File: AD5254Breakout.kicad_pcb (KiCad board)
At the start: 2 copper layers, 20.6 x 18 mm, 13 parts, among them J1 Conn_01x08, J2 Conn_01x08, U1 AD5254

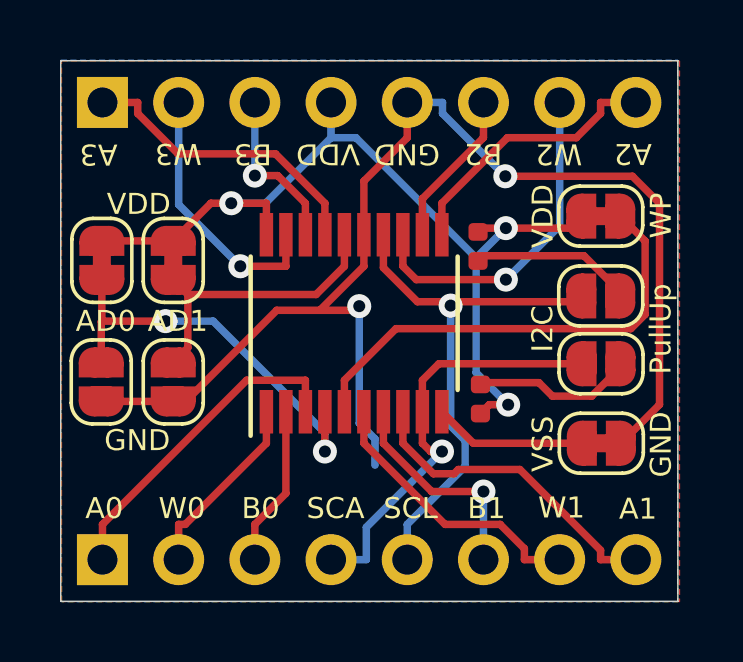
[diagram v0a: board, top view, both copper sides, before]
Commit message: Correct line arround jumper
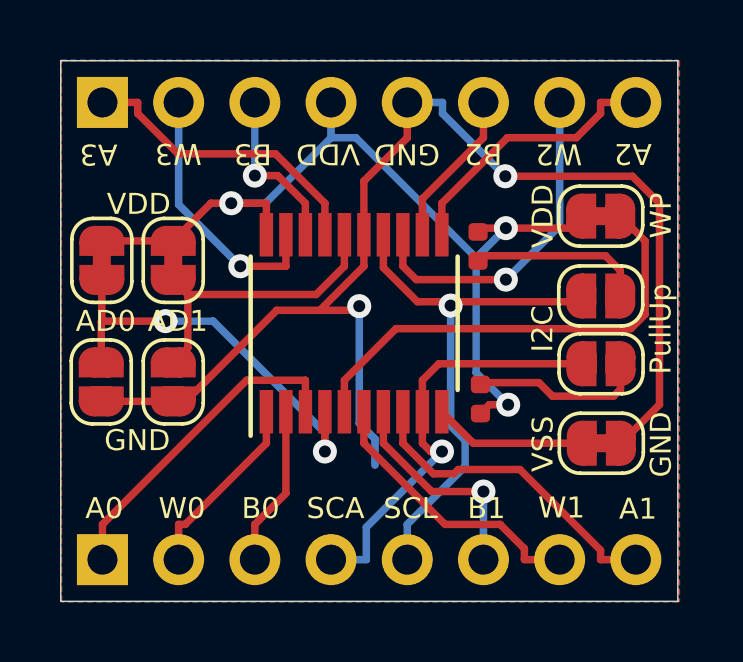
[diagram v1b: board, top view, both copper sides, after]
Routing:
- net Net-(JP8-Pad1): track 5.44 -> 5.99 mm
- net Net-(JP7-Pad1): track 5.40 -> 5.94 mm
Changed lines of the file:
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@@
     (thickness 1.6)
     (drawings 48)
-    (tracks 163)
+    (tracks 165)
     (zones 0)
     (modules 13)
@@
   (segment (start 168.0947 67.7774) (end 168.0947 67.41) (width 0.25) (layer F.Cu) (net 20))
   (segment (start 168.76 76.12) (end 168.76 76.2387) (width 0.25) (layer F.Cu) (net 21))
-  (segment (start 168.76 76.2387) (end 167.7986 77.2001) (width 0.25) (layer F.Cu) (net 21))
-  (segment (start 167.7986 77.2001) (end 166.4902 77.2001) (width 0.25) (layer F.Cu) (net 21))
-  (segment (start 166.4902 77.2001) (end 166.0402 76.7501) (width 0.25) (layer F.Cu) (net 21))
-  (segment (start 166.0402 76.7501) (end 164.1499 76.7501) (width 0.25) (layer F.Cu) (net 21))
-  (segment (start 164.1499 76.7501) (end 164.09 76.81) (width 0.25) (layer F.Cu) (net 21))
+  (segment (start 168.527492 77.2001) (end 168.76 76.967592) (width 0.25) (layer F.Cu) (net 21))
+  (segment (start 166.4902 77.2001) (end 168.527492 77.2001) (width 0.25) (layer F.Cu) (net 21))
+  (segment (start 168.76 76.967592) (end 168.76 76.12) (width 0.25) (layer F.Cu) (net 21))
+  (segment (start 166.0402 76.7501) (end 166.4902 77.2001) (width 0.25) (layer F.Cu) (net 21))
+  (segment (start 164.1499 76.7501) (end 166.0402 76.7501) (width 0.25) (layer F.Cu) (net 21))
+  (segment (start 164.09 76.81) (end 164.1499 76.7501) (width 0.25) (layer F.Cu) (net 21))
   (segment (start 168.75 73.86) (end 168.75 73.7295) (width 0.25) (layer F.Cu) (net 22))
-  (segment (start 168.75 73.7295) (end 167.541 72.5205) (width 0.25) (layer F.Cu) (net 22))
-  (segment (start 167.541 72.5205) (end 164.1845 72.5205) (width 0.25) (layer F.Cu) (net 22))
-  (segment (start 164.1845 72.5205) (end 164.01 72.695) (width 0.25) (layer F.Cu) (net 22))
+  (segment (start 168.75 73.012408) (end 168.75 73.86) (width 0.25) (layer F.Cu) (net 22))
+  (segment (start 168.258092 72.5205) (end 168.75 73.012408) (width 0.25) (layer F.Cu) (net 22))
+  (segment (start 164.1845 72.5205) (end 168.258092 72.5205) (width 0.25) (layer F.Cu) (net 22))
+  (segment (start 164.01 72.695) (end 164.1845 72.5205) (width 0.25) (layer F.Cu) (net 22))
   (zone (net 7) (net_name GND) (layer B.Cu) (hatch edge 0.508)
     (connect_pads (clearance 0.508))
